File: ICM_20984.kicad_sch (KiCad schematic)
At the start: 13 parts, among them Q2 BSS138, Q5 BSS138, U10 ICM-20948, U13 MIC5365-3.3YC5

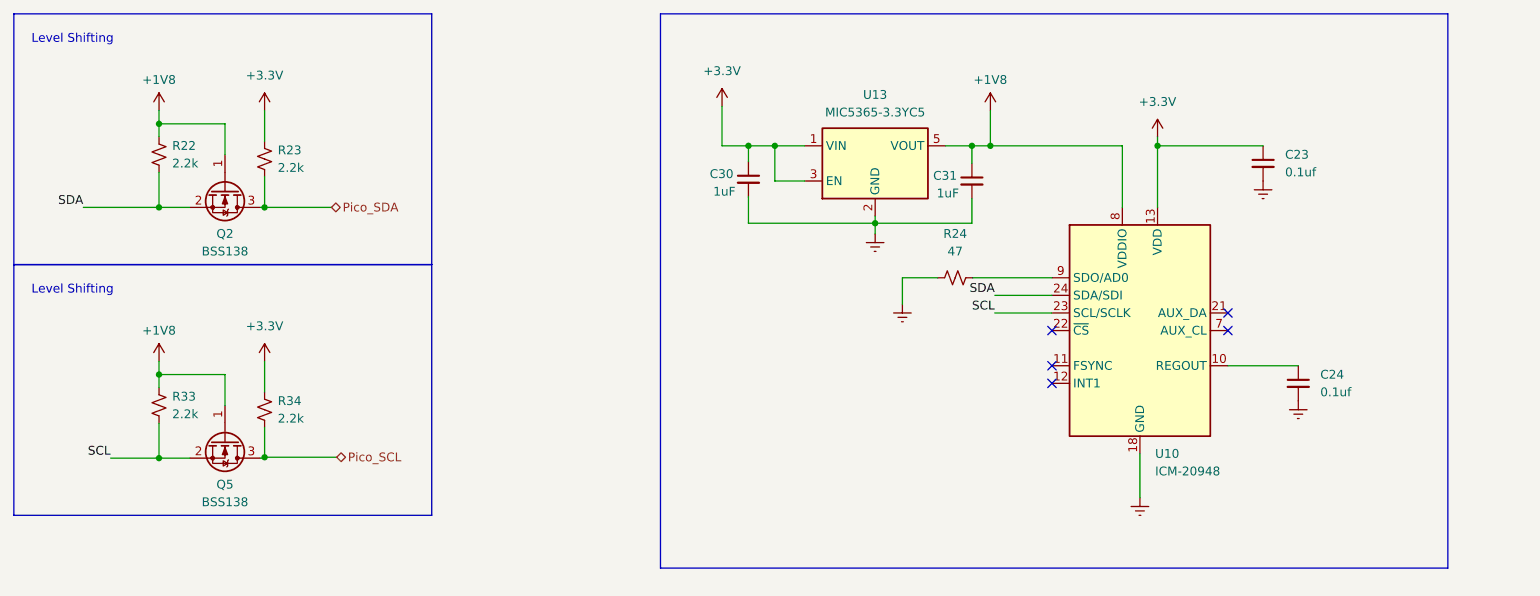
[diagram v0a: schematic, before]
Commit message: clean up Rev
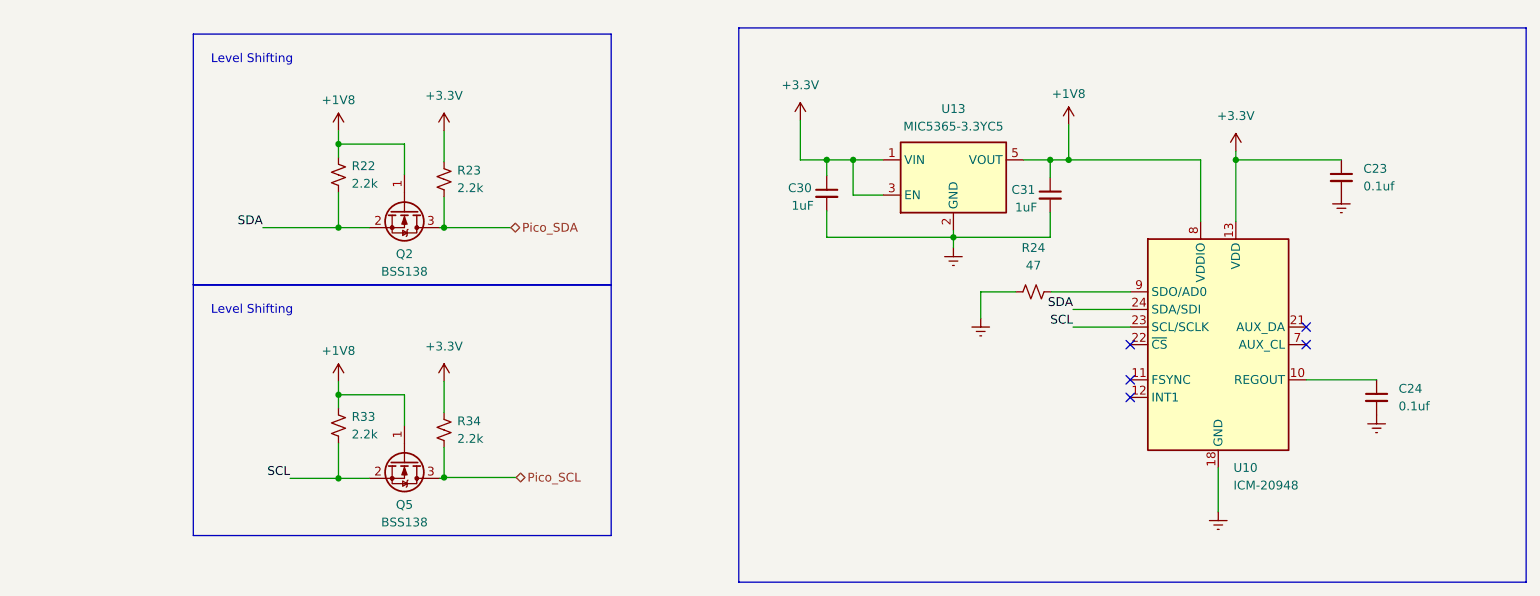
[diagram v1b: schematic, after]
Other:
- moved on the sheet: C23, C24, C30, C31, Q2, Q5, R22, R23, R24, R33, R34, U10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
